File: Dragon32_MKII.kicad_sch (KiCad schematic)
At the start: 223 parts, among them IC1 4116, IC10 SFC2318, IC11 4053, IC12 6847, IC13 74LS273, IC14 74LS86, IC15 74LS783, IC16 74LS244, IC17 ROM8K, IC18 ROM8K, IC19 6809E, IC2 4116, IC20 4529, IC21 74LS123, IC22 74LS00, IC23 74LS74, IC24 74LS244, IC25 LM393, IC26 6821, IC27 74LS20, IC28 74LS393, IC29 74LS393, IC3 4116, IC30 74LS32, IC31 74LS02, IC32 74LS390, IC33 74LS138, IC34 4050, IC35 6821, IC36 4116, IC37 4116, IC38 4116, IC39 4116, IC4 4116, IC40 4116, IC41 4116, IC42 4116, IC43 4116, IC5 4116, IC6 4116, IC7 4116, IC8 4116, IC9 LM1889, SW1 RESET, U1 LINE_PULSE_DIAGRAM

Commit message: refine component locations
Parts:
- D1, D10, D2, D3, D4, D5, D6, D7, D8, D9: footprint Diode_THT:D_DO-35_SOD27_P7.62mm_Horizontal -> Diode_THT:D_DO-35_SOD27_P12.70mm_Horizontal
- L1, L2: footprint Inductor_THT:L_Axial_L7.0mm_D3.3mm_P10.16mm_Horizontal_Fastron_MICC -> Inductor_THT:L_Axial_L7.0mm_D3.3mm_P12.70mm_Horizontal_Fastron_MICC
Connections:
- net +5V: now also R36.2, R39.2, R49.2, R50.2, R52.2, R63.2; no longer R36.1, R39.1, R49.1, R50.1, R52.1, R63.1
- net A7: now also R74.2; no longer R74.1
- net BITSND: now also R56.1; no longer R56.2
- net CASIN: now also R49.1, R51.2; no longer R49.2, R51.1
- net GND: now also R46.1, R74.1; no longer R46.2, R74.2
- net SOUND: now also R56.2; no longer R56.1
- net ~{CART}: now also R63.1; no longer R63.2
- net ~{EXTMEM}: now also R39.1; no longer R39.2
- net at C4.1, D4.2 (K), D5.2 (K)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: now also R36.1; no longer R36.2
- net at IC25.2 (_), R45.2: now also R52.1; no longer R52.2
- net at IC25.3 (+), R48.1: now also R50.1, R51.1; no longer R50.2, R51.2
- net at C35.2, C44.1, R47.1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: now also R46.2; no longer R46.1
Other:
- moved on the sheet: R49, R51
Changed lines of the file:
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@@
       (effects (font (size 1.27 1.27)) (justify left))
     )
-    (property "Footprint" "Diode_THT:D_DO-35_SOD27_P7.62mm_Horizontal" (at 45.72 115.57 0)
+    (property "Footprint" "Diode_THT:D_DO-35_SOD27_P12.70mm_Horizontal" (at 45.72 115.57 0)
       (effects (font (size 1.524 1.524)) hide)
     )
@@
     )
   )
-  (symbol (lib_id "Dragon32_MKII:R") (at 57.15 115.57 0) (unit 1)
+  (symbol (lib_id "Dragon32_MKII:R") (at 57.15 115.57 0) (mirror x) (unit 1)
     (in_bom yes) (on_board yes) (dnp no)
-    (property "Reference" "R36" (at 59.69 114.3 0)
+    (property "Reference" "R36" (at 59.69 116.84 0)
       (effects (font (size 1.27 1.27)) (justify left))
     )
-    (property "Value" "100K" (at 59.69 116.84 0)
+    (property "Value" "100K" (at 59.69 114.3 0)
       (effects (font (size 1.27 1.27)) (justify left))
     )
@@
     )
   )
-  (symbol (lib_id "Dragon32_MKII:R") (at 30.48 92.71 0) (unit 1)
+  (symbol (lib_id "Dragon32_MKII:R") (at 30.48 92.71 0) (mirror x) (unit 1)
     (in_bom yes) (on_board yes) (dnp yes)
-    (property "Reference" "R74" (at 33.02 91.44 0)
+    (property "Reference" "R74" (at 33.02 93.98 0)
       (effects (font (size 1.27 1.27)) (justify left))
     )
-    (property "Value" "Not Fitted" (at 33.02 93.98 0)
+    (property "Value" "Not Fitted" (at 33.02 91.44 0)
       (effects (font (size 1.27 1.27)) (justify left))
     )
@@
       (effects (font (size 1.27 1.27)) (justify left))
     )
-    (property "Footprint" "Diode_THT:D_DO-35_SOD27_P7.62mm_Horizontal" (at 44.45 92.71 0)
+    (property "Footprint" "Diode_THT:D_DO-35_SOD27_P12.70mm_Horizontal" (at 44.45 92.71 0)
       (effects (font (size 1.524 1.524)) hide)
     )
@@
       (effects (font (size 1.27 1.27)) (justify left))
     )
-    (property "Footprint" "Diode_THT:D_DO-35_SOD27_P7.62mm_Horizontal" (at 30.48 129.54 0)
+    (property "Footprint" "Diode_THT:D_DO-35_SOD27_P12.70mm_Horizontal" (at 30.48 129.54 0)
       (effects (font (size 1.524 1.524)) hide)
     )
@@
       (effects (font (size 1.27 1.27)) (justify left))
     )
-    (property "Footprint" "Diode_THT:D_DO-35_SOD27_P7.62mm_Horizontal" (at 30.48 111.76 0)
+    (property "Footprint" "Diode_THT:D_DO-35_SOD27_P12.70mm_Horizontal" (at 30.48 111.76 0)
       (effects (font (size 1.524 1.524)) hide)
     )
@@
     )
   )
-  (symbol (lib_id "Dragon32_MKII:R") (at 243.84 86.36 0) (unit 1)
+  (symbol (lib_id "Dragon32_MKII:R") (at 243.84 86.36 0) (mirror x) (unit 1)
     (in_bom yes) (on_board yes) (dnp no)
-    (property "Reference" "R39" (at 246.38 85.09 0)
+    (property "Reference" "R39" (at 246.38 87.63 0)
       (effects (font (size 1.27 1.27)) (justify left))
     )
-    (property "Value" "4K7" (at 246.38 87.63 0)
+    (property "Value" "4K7" (at 246.38 85.09 0)
       (effects (font (size 1.27 1.27)) (justify left))
     )
@@
       (effects (font (size 1.27 1.27)))
     )
-    (property "Footprint" "Inductor_THT:L_Axial_L7.0mm_D3.3mm_P10.16mm_Horizontal_Fastron_MICC" (at 652.78 64.77 0)
+    (property "Footprint" "Inductor_THT:L_Axial_L7.0mm_D3.3mm_P12.70mm_Horizontal_Fastron_MICC" (at 652.78 64.77 0)
       (effects (font (size 1.524 1.524)) hide)
     )
@@
       (effects (font (size 1.27 1.27)))
     )
-    (property "Footprint" "Inductor_THT:L_Axial_L7.0mm_D3.3mm_P10.16mm_Horizontal_Fastron_MICC" (at 652.78 95.25 0)
+    (property "Footprint" "Inductor_THT:L_Axial_L7.0mm_D3.3mm_P12.70mm_Horizontal_Fastron_MICC" (at 652.78 95.25 0)
       (effects (font (size 1.524 1.524)) hide)
     )
@@
     )
   )
-  (symbol (lib_id "Dragon32_MKII:R") (at 473.71 156.21 0) (unit 1)
+  (symbol (lib_id "Dragon32_MKII:R") (at 473.71 156.21 0) (mirror x) (unit 1)
     (in_bom yes) (on_board yes) (dnp no)
-    (property "Reference" "R63" (at 477.52 154.94 0)
+    (property "Reference" "R63" (at 477.52 157.48 0)
       (effects (font (size 1.27 1.27)))
     )
-    (property "Value" "4K7" (at 477.52 157.48 0)
+    (property "Value" "4K7" (at 477.52 154.94 0)
       (effects (font (size 1.27 1.27)))
     )
@@
     )
   )
-  (symbol (lib_id "Dragon32_MKII:R") (at 742.95 92.71 0) (unit 1)
+  (symbol (lib_id "Dragon32_MKII:R") (at 742.95 92.71 0) (mirror x) (unit 1)
     (in_bom yes) (on_board yes) (dnp no)
-    (property "Reference" "R56" (at 746.76 91.44 0)
+    (property "Reference" "R56" (at 746.76 93.98 0)
       (effects (font (size 1.27 1.27)))
     )
-    (property "Value" "10K" (at 746.76 93.98 0)
+    (property "Value" "10K" (at 746.76 91.44 0)
       (effects (font (size 1.27 1.27)))
     )
@@
     )
   )
-  (symbol (lib_id "Dragon32_MKII:R") (at 772.16 160.02 270) (unit 1)
+  (symbol (lib_id "Dragon32_MKII:R") (at 772.16 160.02 90) (mirror x) (unit 1)
     (in_bom yes) (on_board yes) (dnp no)
     (property "Reference" "R51" (at 772.16 154.94 90)
@@
     )
   )
-  (symbol (lib_id "Dragon32_MKII:R") (at 786.13 154.94 0) (unit 1)
+  (symbol (lib_id "Dragon32_MKII:R") (at 786.13 154.94 180) (unit 1)
     (in_bom yes) (on_board yes) (dnp no)
-    (property "Reference" "R49" (at 789.94 153.67 0)
+    (property "Reference" "R49" (at 782.32 156.21 0)
       (effects (font (size 1.27 1.27)))
     )
-    (property "Value" "1K" (at 789.94 156.21 0)
+    (property "Value" "1K" (at 782.32 153.67 0)
       (effects (font (size 1.27 1.27)))
     )
-    (property "Footprint" "Dragon:R_Axial_DIN0207_L6.3mm_D2.5mm_P12.7mm_Horizontal" (at 784.352 154.94 90)
+    (property "Footprint" "Dragon:R_Axial_DIN0207_L6.3mm_D2.5mm_P12.7mm_Horizontal" (at 787.908 154.94 90)
       (effects (font (size 0.762 0.762)) hide)
     )
@@
     )
   )
-  (symbol (lib_id "Dragon32_MKII:R") (at 758.19 154.94 0) (unit 1)
+  (symbol (lib_id "Dragon32_MKII:R") (at 758.19 154.94 0) (mirror x) (unit 1)
     (in_bom yes) (on_board yes) (dnp no)
-    (property "Reference" "R50" (at 762 153.67 0)
+    (property "Reference" "R50" (at 762 156.21 0)
       (effects (font (size 1.27 1.27)))
     )
-    (property "Value" "56K" (at 762 156.21 0)
+    (property "Value" "56K" (at 762 153.67 0)
       (effects (font (size 1.27 1.27)))
     )
@@
     )
   )
-  (symbol (lib_id "Dragon32_MKII:R") (at 748.03 162.56 0) (unit 1)
+  (symbol (lib_id "Dragon32_MKII:R") (at 748.03 162.56 0) (mirror x) (unit 1)
     (in_bom yes) (on_board yes) (dnp no)
-    (property "Reference" "R52" (at 751.84 161.29 0)
+    (property "Reference" "R52" (at 751.84 163.83 0)
       (effects (font (size 1.27 1.27)))
     )
-    (property "Value" "56K" (at 751.84 163.83 0)
+    (property "Value" "56K" (at 751.84 161.29 0)
       (effects (font (size 1.27 1.27)))
     )
@@
       (effects (font (size 1.27 1.27)) (justify left))
     )
-    (property "Footprint" "Diode_THT:D_DO-35_SOD27_P7.62mm_Horizontal" (at 638.81 152.4 0)
+    (property "Footprint" "Diode_THT:D_DO-35_SOD27_P12.70mm_Horizontal" (at 638.81 152.4 0)
       (effects (font (size 1.524 1.524)) hide)
     )
@@
       (effects (font (size 1.27 1.27)))
     )
-    (property "Footprint" "Diode_THT:D_DO-35_SOD27_P7.62mm_Horizontal" (at 665.48 149.86 0)
+    (property "Footprint" "Diode_THT:D_DO-35_SOD27_P12.70mm_Horizontal" (at 665.48 149.86 0)
       (effects (font (size 1.524 1.524)) hide)
     )
@@
       (effects (font (size 1.27 1.27)))
     )
-    (property "Footprint" "Diode_THT:D_DO-35_SOD27_P7.62mm_Horizontal" (at 665.48 154.94 0)
+    (property "Footprint" "Diode_THT:D_DO-35_SOD27_P12.70mm_Horizontal" (at 665.48 154.94 0)
       (effects (font (size 1.524 1.524)) hide)
     )
@@
     )
   )
-  (symbol (lib_id "Dragon32_MKII:R") (at 708.66 182.88 0) (unit 1)
+  (symbol (lib_id "Dragon32_MKII:R") (at 708.66 182.88 0) (mirror x) (unit 1)
     (in_bom yes) (on_board yes) (dnp no)
-    (property "Reference" "R46" (at 712.47 181.61 0)
+    (property "Reference" "R46" (at 712.47 184.15 0)
       (effects (font (size 1.27 1.27)))
     )
-    (property "Value" "220R" (at 712.47 184.15 0)
+    (property "Value" "220R" (at 712.47 181.61 0)
       (effects (font (size 1.27 1.27)))
     )
@@
       (effects (font (size 1.27 1.27)) (justify left))
     )
-    (property "Footprint" "Diode_THT:D_DO-35_SOD27_P7.62mm_Horizontal" (at 735.33 181.61 0)
+    (property "Footprint" "Diode_THT:D_DO-35_SOD27_P12.70mm_Horizontal" (at 735.33 181.61 0)
       (effects (font (size 1.524 1.524)) hide)
     )
@@
       (effects (font (size 1.27 1.27)) (justify left))
     )
-    (property "Footprint" "Diode_THT:D_DO-35_SOD27_P7.62mm_Horizontal" (at 730.25 203.2 0)
+    (property "Footprint" "Diode_THT:D_DO-35_SOD27_P12.70mm_Horizontal" (at 730.25 203.2 0)
       (effects (font (size 1.524 1.524)) hide)
     )
@@
       (effects (font (size 1.27 1.27)) (justify left))
     )
-    (property "Footprint" "Diode_THT:D_DO-35_SOD27_P7.62mm_Horizontal" (at 730.25 214.63 0)
+    (property "Footprint" "Diode_THT:D_DO-35_SOD27_P12.70mm_Horizontal" (at 730.25 214.63 0)
       (effects (font (size 1.524 1.524)) hide)
     )

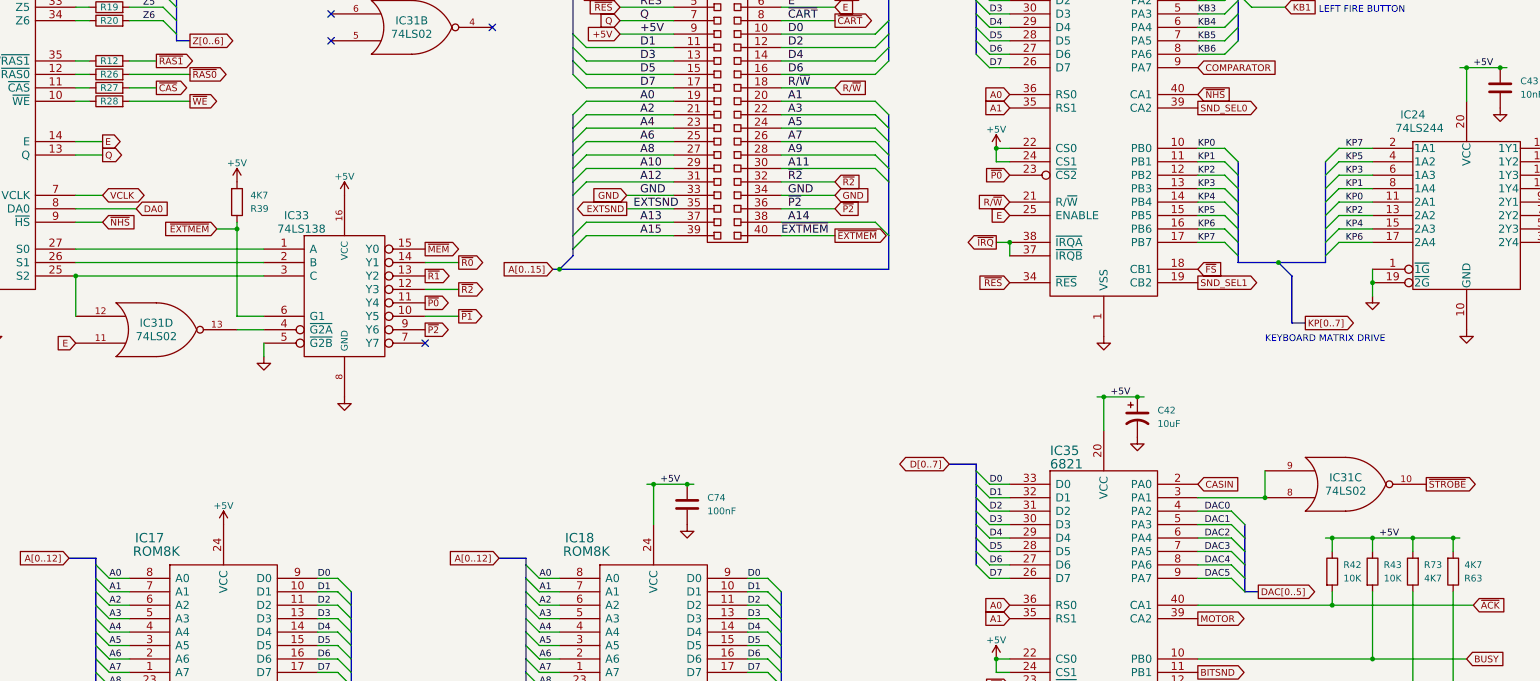
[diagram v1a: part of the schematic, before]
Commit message: trace routes
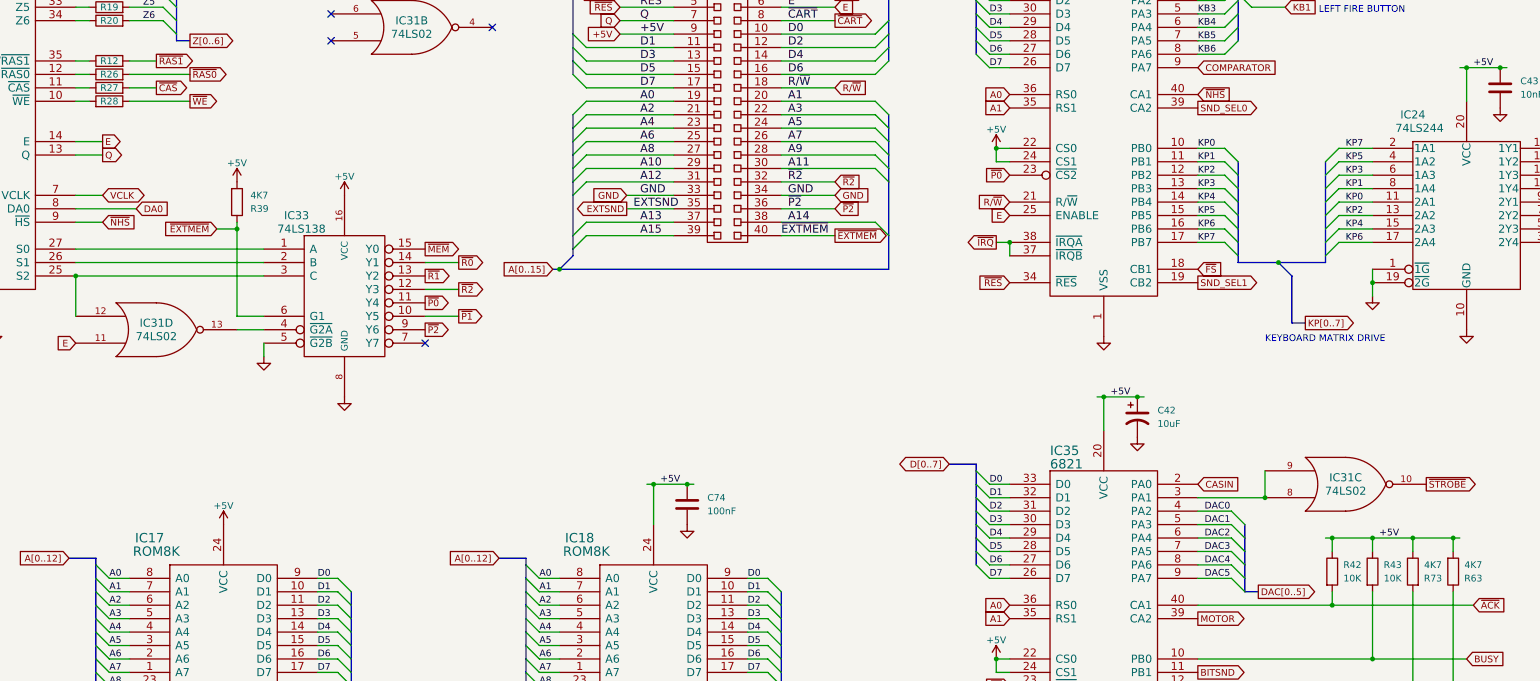
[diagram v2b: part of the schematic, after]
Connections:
- net +5V: now also R73.1; no longer R73.2
- net ~{WE}: now also R28.1; no longer R28.2
- net at IC15.10 (~{WE}): now also R28.2; no longer R28.1
- net at IC35.12 (PB2): now also R73.2; no longer R73.1
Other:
- moved on the sheet: R28, R73
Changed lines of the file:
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@@
     )
   )
-  (symbol (lib_id "Dragon32_MKII:R") (at 219.71 67.31 90) (unit 1)
+  (symbol (lib_id "Dragon32_MKII:R") (at 219.71 67.31 270) (mirror x) (unit 1)
     (in_bom yes) (on_board yes) (dnp no)
     (property "Reference" "R28" (at 219.71 67.31 90)
       (effects (font (size 1.27 1.27)))
     )
-    (property "Value" "22R" (at 228.6 66.04 90)
+    (property "Value" "22R" (at 210.82 66.04 90)
       (effects (font (size 1.27 1.27)) (justify left) hide)
     )
@@
     )
   )
-  (symbol (lib_id "Dragon32_MKII:R") (at 466.09 156.21 180) (unit 1)
+  (symbol (lib_id "Dragon32_MKII:R") (at 466.09 156.21 0) (mirror y) (unit 1)
     (in_bom yes) (on_board yes) (dnp no)
-    (property "Reference" "R73" (at 469.9 154.94 0)
+    (property "Reference" "R73" (at 469.9 157.48 0)
       (effects (font (size 1.27 1.27)))
     )
-    (property "Value" "4K7" (at 469.9 157.48 0)
+    (property "Value" "4K7" (at 469.9 154.94 0)
       (effects (font (size 1.27 1.27)))
     )
